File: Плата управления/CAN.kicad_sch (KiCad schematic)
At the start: 8 parts

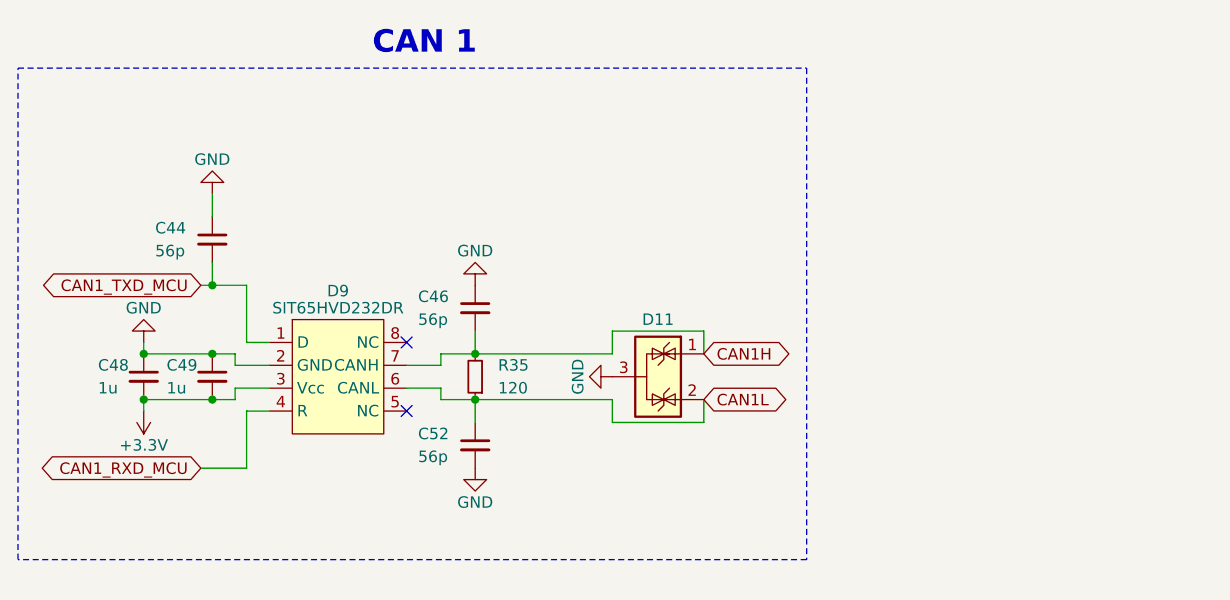
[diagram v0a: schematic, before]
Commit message: Изменения: добавил папку с отчетностью
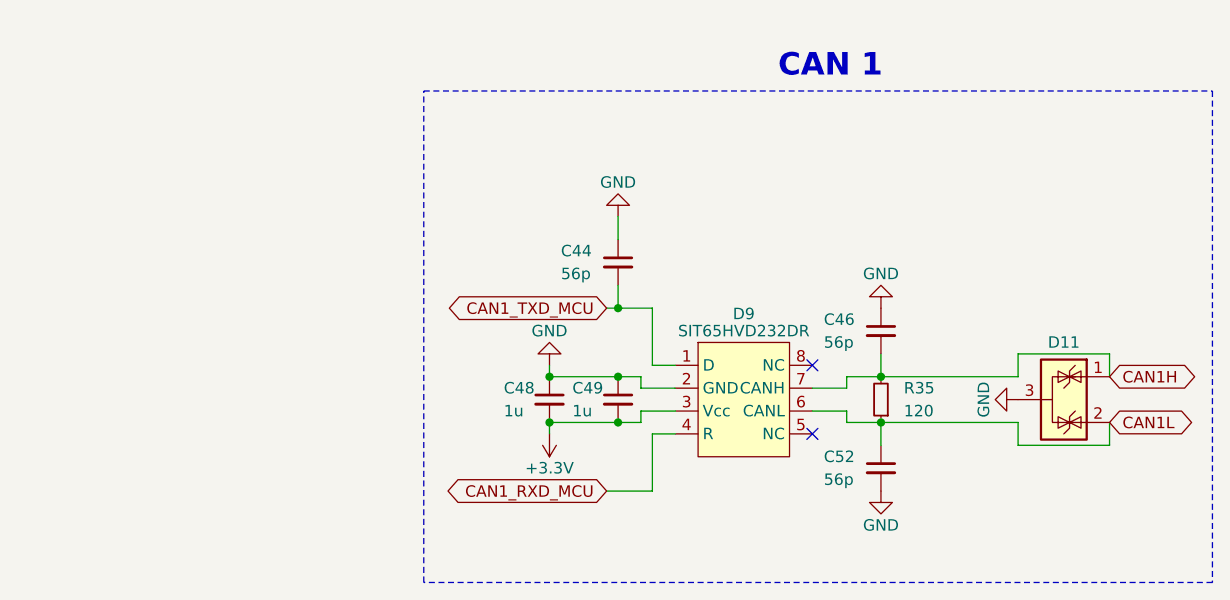
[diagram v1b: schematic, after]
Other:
- moved on the sheet: C44, C46, C48, C49, C52, D11, D9, R35
